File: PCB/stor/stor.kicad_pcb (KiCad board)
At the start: 4 copper layers, 22 x 58.8 mm, 56 parts, among them J1 Conn_01x05_Socket, J2 Conn_01x04_Socket, SW1 TS1603-TZ38HBM, SW2 TS1603-TZ38HBM, U1 STM32H723VGT6, U3 USB3300-EZK-TR, U4 TPS62177DQCR, X1 25mhz, X2 32.768k, X3 24mhz

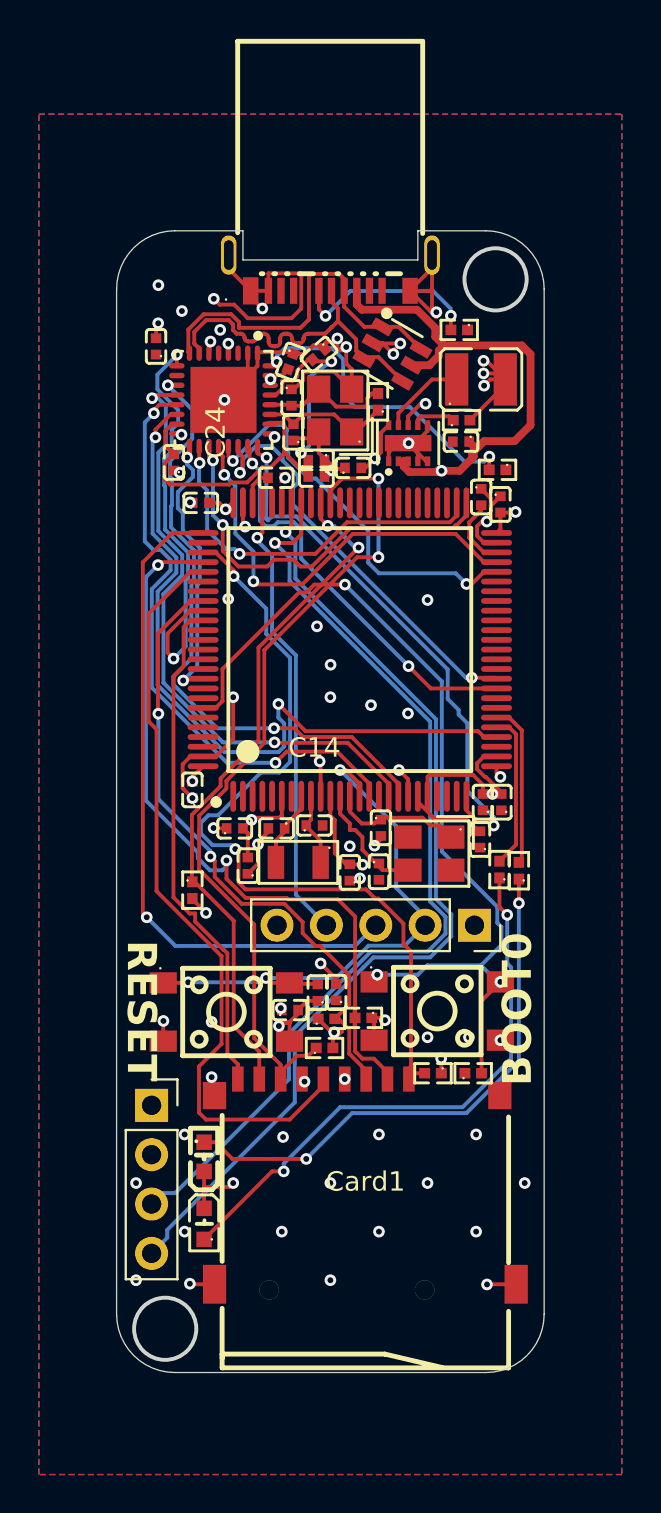
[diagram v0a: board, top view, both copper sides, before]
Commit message: Update stor.kicad_pcb
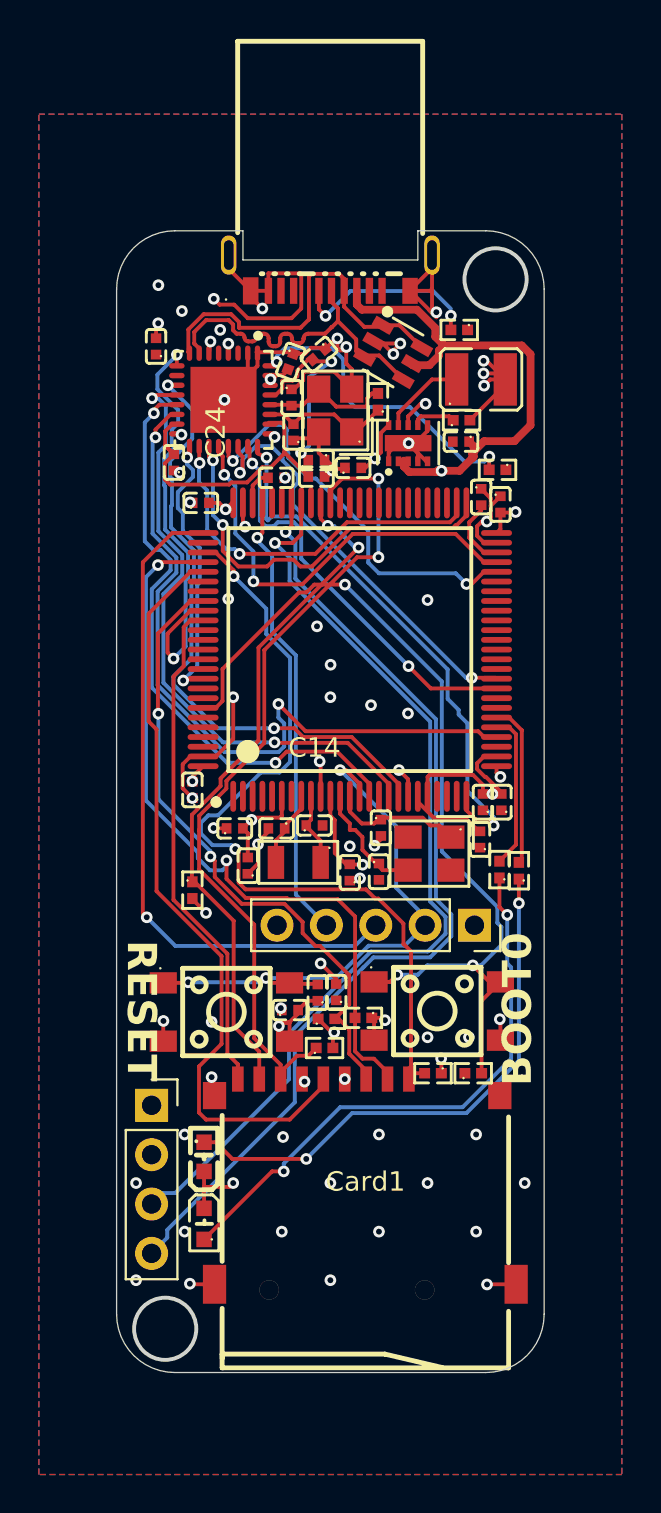
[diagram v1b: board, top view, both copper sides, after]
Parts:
- moved D1 0.09 mm to (123.2, 42.3)
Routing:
- net /PC11: track 39.4 -> 38.5 mm
- net /BOOT0: track 45.6 -> 46.3 mm
- net /VDD: track 51.6 -> 50.9 mm
